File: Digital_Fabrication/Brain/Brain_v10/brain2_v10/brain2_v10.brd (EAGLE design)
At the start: 140.7 x 108 mm, 86 parts

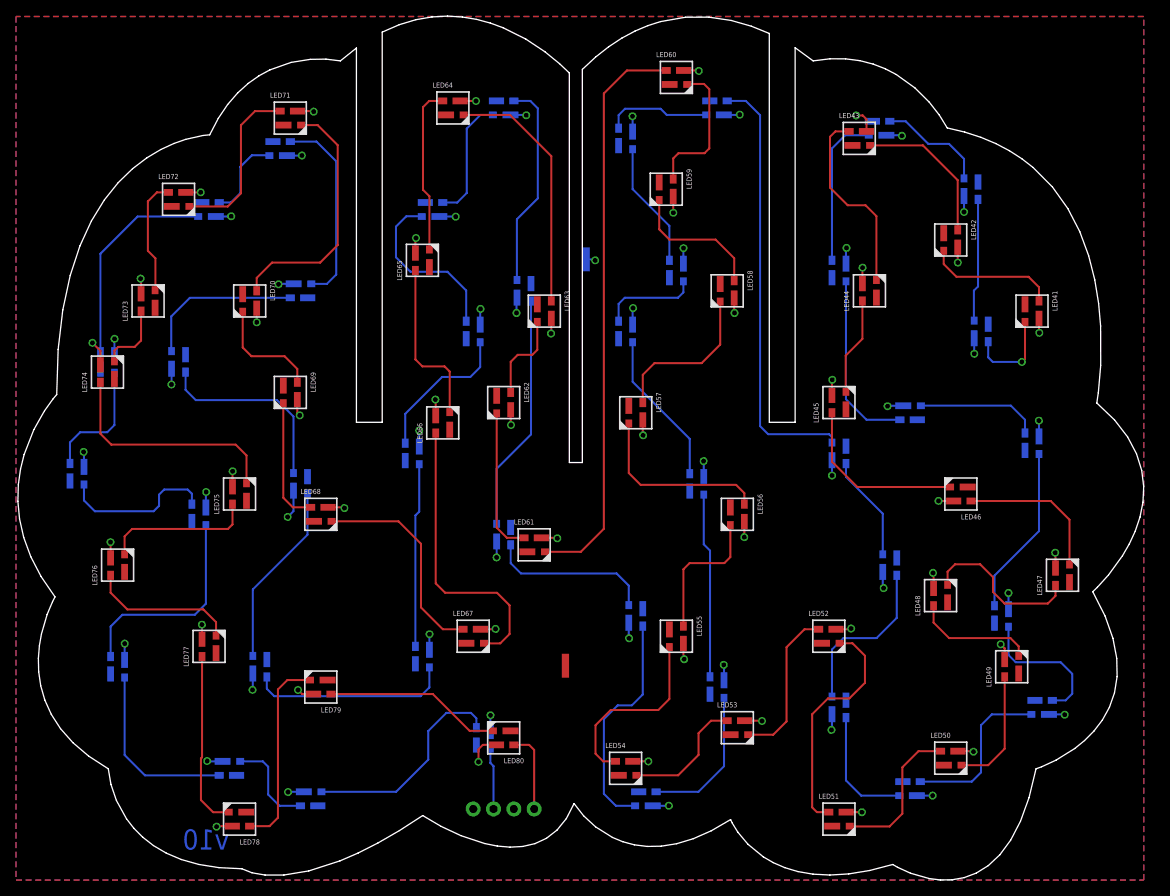
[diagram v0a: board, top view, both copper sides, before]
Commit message: generate gerbers
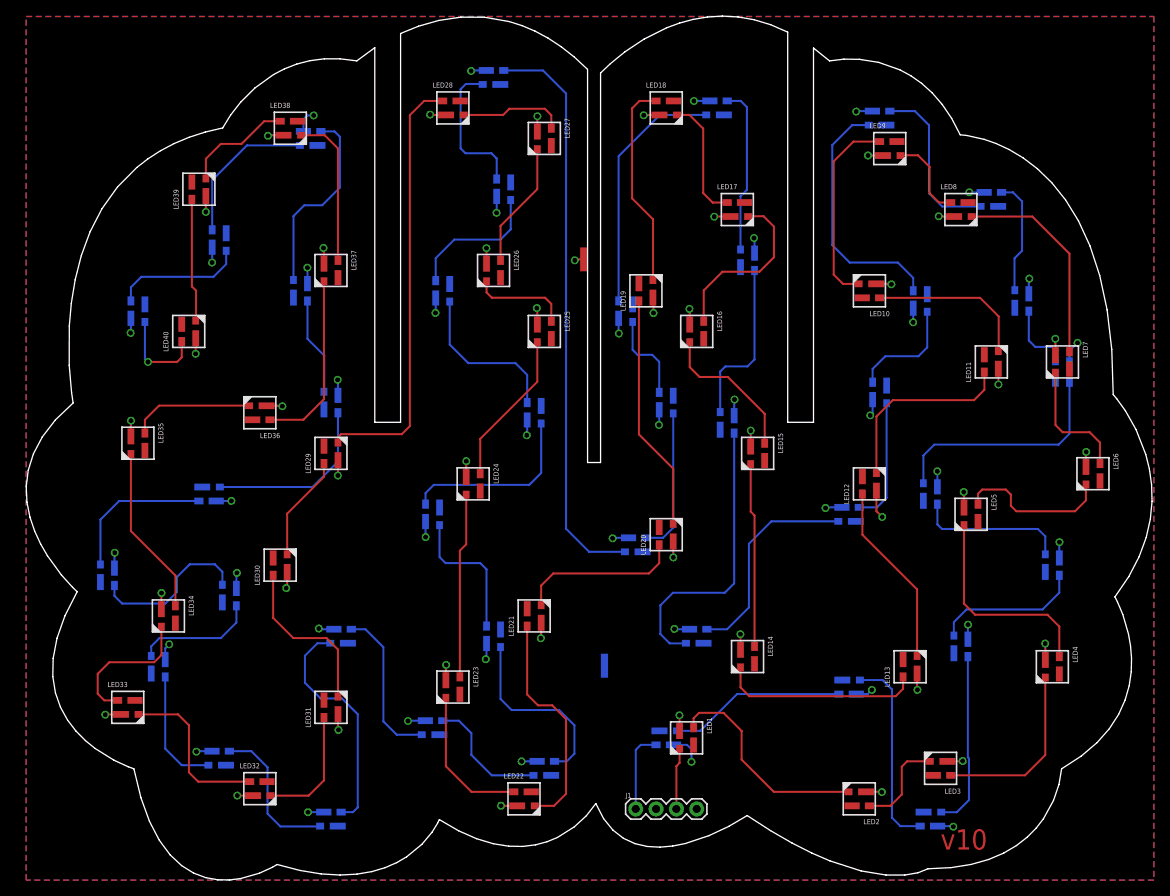
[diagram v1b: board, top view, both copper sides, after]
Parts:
- moved FRAME1 299.7 mm to (-80.0, 1.27), flipped to the top
- moved FRAME2 299.7 mm to (-80.0, 10.2), flipped to the top
- moved FRAME3 299.7 mm to (-80.0, 19.1), flipped to the top
- moved LED6 127.0 mm to (133.3, 50.8), flipped to the top
- moved LED47 119.4 mm to (10.2, 38.1), flipped to the bottom
- moved LED7 119.4 mm to (129.5, 64.8), flipped to the top
- moved LED74 119.4 mm to (129.5, 63.5), flipped to the bottom
- moved LED4 116.8 mm to (128.3, 26.7), flipped to the top
- moved LED76 116.8 mm to (128.3, 39.4), flipped to the bottom
- moved LED33 114.3 mm to (12.7, 21.6), flipped to the top
- moved LED35 111.8 mm to (14.0, 54.6), flipped to the top
- moved LED41 111.8 mm to (14.0, 71.1), flipped to the bottom
- moved LED73 109.2 mm to (124.5, 72.4), flipped to the bottom
- moved LED49 106.7 mm to (16.5, 26.7), flipped to the bottom
- moved LED34 104.1 mm to (17.8, 33.0), flipped to the top
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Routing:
- added copper zone on layer 1, net 5V
- added copper zone on layer 16, net GND
- removed copper zone on layer 16, net 5V
- removed copper zone on layer 1, net GND
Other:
- outline, holes or cut-outs redrawn
